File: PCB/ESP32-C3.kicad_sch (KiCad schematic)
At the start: 28 parts, among them J1 HCZZ0039-3, J2 DPS_PPS_Right_Angle, SW2 TS4535TP 250gf 009, U1 USB-C-16P-SMD, U3 ESP32-C3, Y1 40MHz_S3240000151040

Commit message: updated
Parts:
- AE1: footprint Resistor_SMD:R_1206_3216Metric -> RF_Antenna:Texas_SWRA117D_2.4GHz_Left
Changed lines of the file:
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@@
 			)
 		)
-		(property "Footprint" "Resistor_SMD:R_1206_3216Metric"
+		(property "Footprint" "RF_Antenna:Texas_SWRA117D_2.4GHz_Left"
 			(at 82.55 92.71 0)
 			(effects

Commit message: Zur Kontrolle fertig.
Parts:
- J2: LCSC C5368738 -> C7465576
- U3: LCSC C2848860 -> C5143572
- Y1: LCSC C426990 -> C5261247
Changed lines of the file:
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@@
 			)
 		)
-		(property "LCSC" "C5368738"
+		(property "LCSC" "C7465576"
 			(at 81.28 36.83 0)
 			(effects
@@
 			)
 		)
-		(property "LCSC" "C426990"
+		(property "LCSC" "C5261247"
 			(at 217.17 116.84 0)
 			(effects
@@
 			)
 		)
-		(property "LCSC" "C2848860"
+		(property "LCSC" "C5143572"
 			(at 133.35 105.41 0)
 			(effects

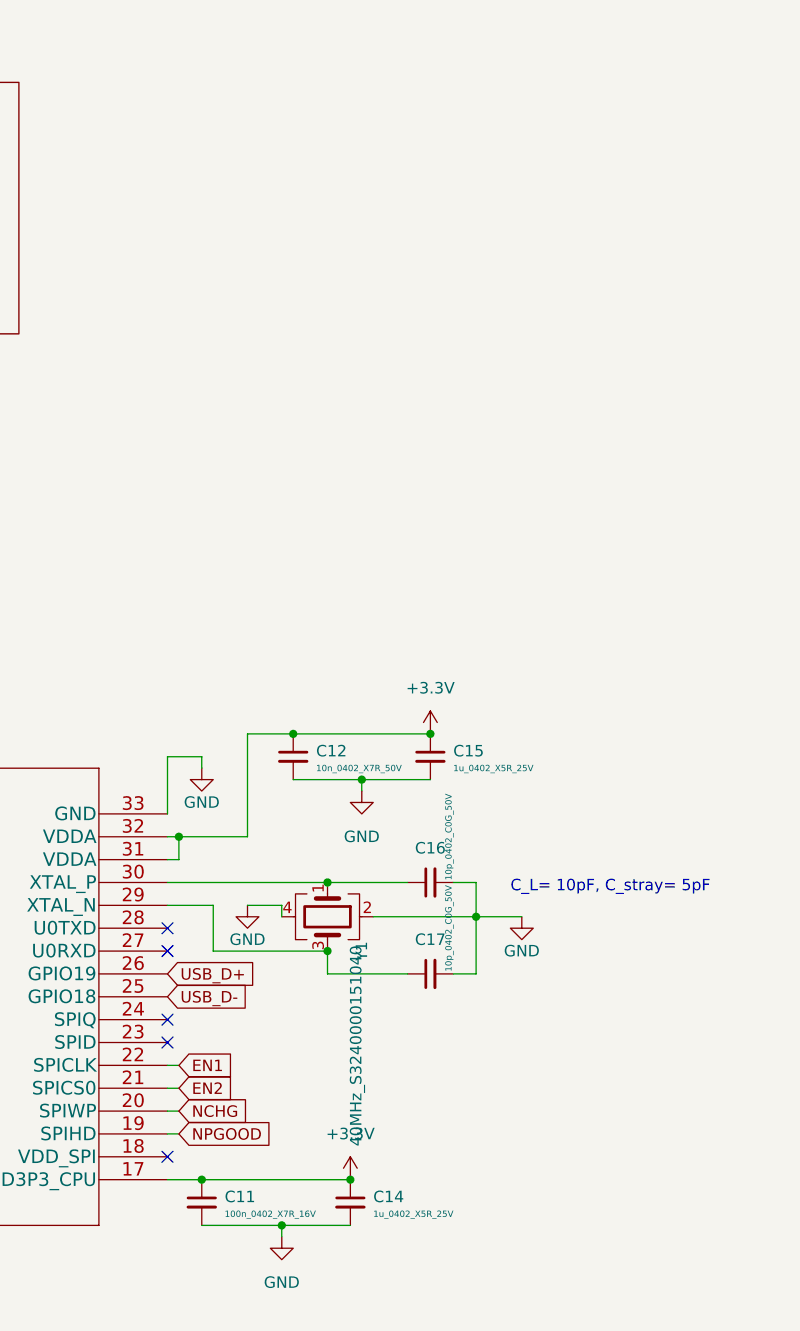
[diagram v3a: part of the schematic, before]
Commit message: Neuste Version
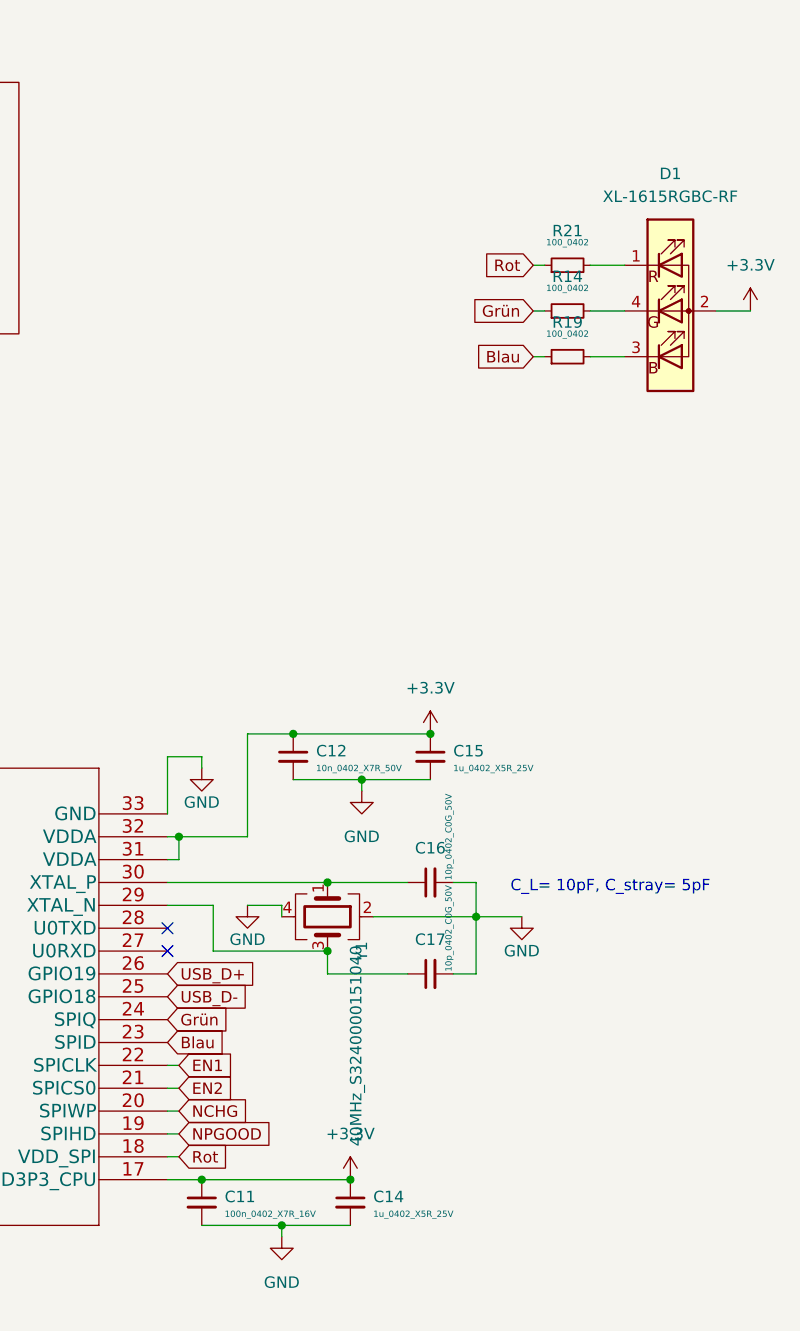
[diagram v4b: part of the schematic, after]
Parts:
- added D1: XL-1615RGBC-RF, LEDSMD:LED_0606_1432, symbol led:XL-1615RGBC-RF
- added R14, R19, R21: 100_0402, Resistor_SMD:R_0402_1005Metric, symbol resistor_smd_standard:100_0402
- U3: LCSC C5143572 -> C2858491
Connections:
- net +3.3V: now also D1.2 (A)
- net Rot: now reaches U3.18 (VDD_SPI)
- net Rot: now also R21.1
- net Blau: now reaches U3.23 (SPID)
- net Blau: now also R19.1
- net Grün: now reaches U3.24 (SPIQ)
- net Grün: now also R14.1
- new net: D1.3 (BK), R19.2
- new net: D1.1 (RK), R21.2
- new net: D1.4 (GK), R14.2
- no-connect marks 20 -> 17
